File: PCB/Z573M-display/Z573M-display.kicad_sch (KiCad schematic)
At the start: 59 parts, among them J1 OSTVN02A150, J2 OSTVN02A150, J4 Conn_01x05_Socket, J5 Conn_01x06_Socket, Q1 MPSA92, Q10 MPSA42, Q11 MPSA42, Q12 MPSA42, Q13 MPSA42, Q2 MPSA92, Q3 MPSA92, Q4 MPSA42, Q5 MPSA42, Q6 MPSA42, Q7 MPSA92, Q8 MPSA92, Q9 MPSA92, U1 74141, U2 Z573M_Board, U3 Z573M_Board, U4 Z573M_Board, U5 Z573M_Board, U6 Z573M_Board, U7 Z573M_Board

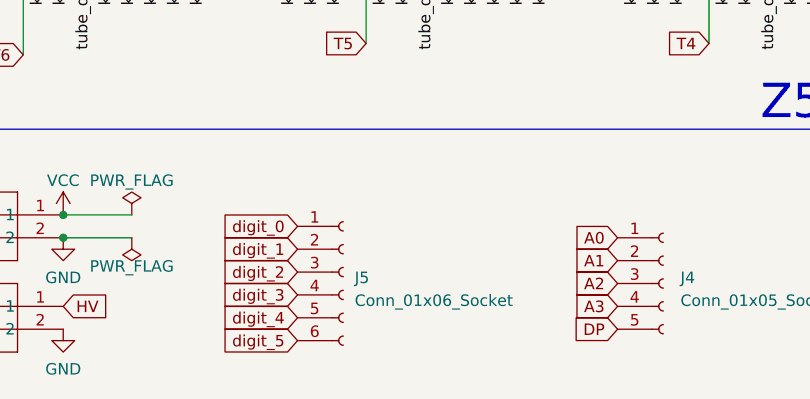
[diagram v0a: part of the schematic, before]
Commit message: Horizontal pins
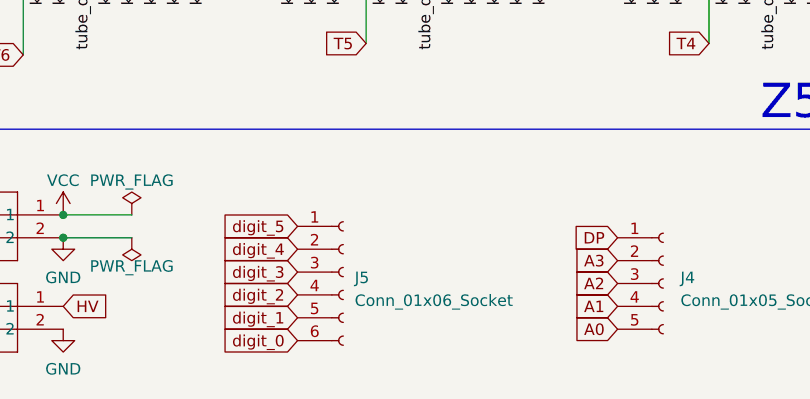
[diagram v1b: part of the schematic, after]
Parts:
- J4: footprint nixie-2.1-footprints:PinHeader_1x05_P2.54mm_Vertical -> Connector_PinHeader_2.54mm:PinHeader_1x05_P2.54mm_Horizontal
- J5: footprint nixie-2.1-footprints:PinHeader_1x06_P2.54mm_Vertical -> Connector_PinHeader_2.54mm:PinHeader_1x06_P2.54mm_Horizontal
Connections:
- net A0: now also J4.5 (Pin_5); no longer J4.1 (Pin_1)
- net A1: now also J4.4 (Pin_4); no longer J4.2 (Pin_2)
- net A3: now also J4.2 (Pin_2); no longer J4.4 (Pin_4)
- net DP: now also J4.1 (Pin_1); no longer J4.5 (Pin_5)
- net digit_0: now also J5.6 (Pin_6); no longer J5.1 (Pin_1)
- net digit_1: now also J5.5 (Pin_5); no longer J5.2 (Pin_2)
- net digit_2: now also J5.4 (Pin_4); no longer J5.3 (Pin_3)
- net digit_3: now also J5.3 (Pin_3); no longer J5.4 (Pin_4)
- net digit_4: now also J5.2 (Pin_2); no longer J5.5 (Pin_5)
- net digit_5: now also J5.1 (Pin_1); no longer J5.6 (Pin_6)
